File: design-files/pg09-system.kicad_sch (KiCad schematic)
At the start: 15 parts, among them U101 MC6809E, U102 GAL22V10, U103 74AHCT245, U104 74AHCT245, U105 74AHCT245, U106 GAL22V10

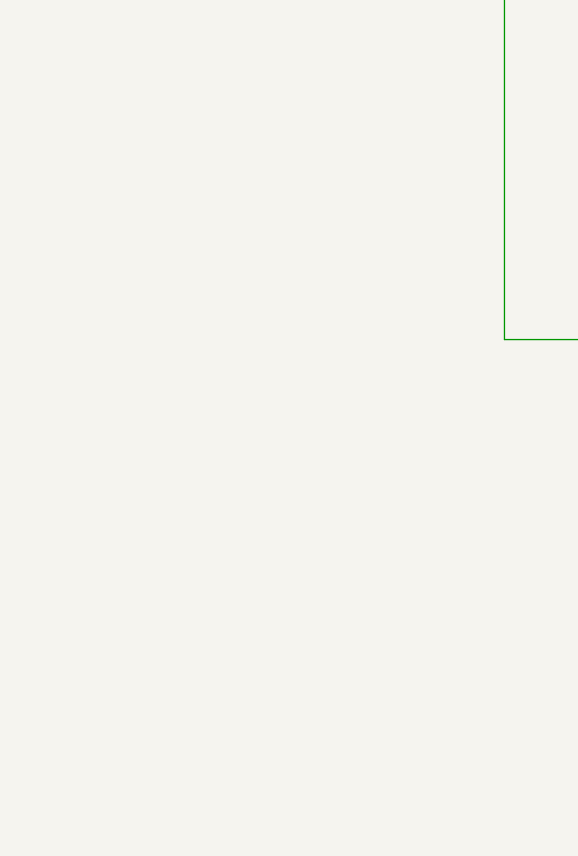
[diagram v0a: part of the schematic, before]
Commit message: Checkpoint WIP new PCB layout.
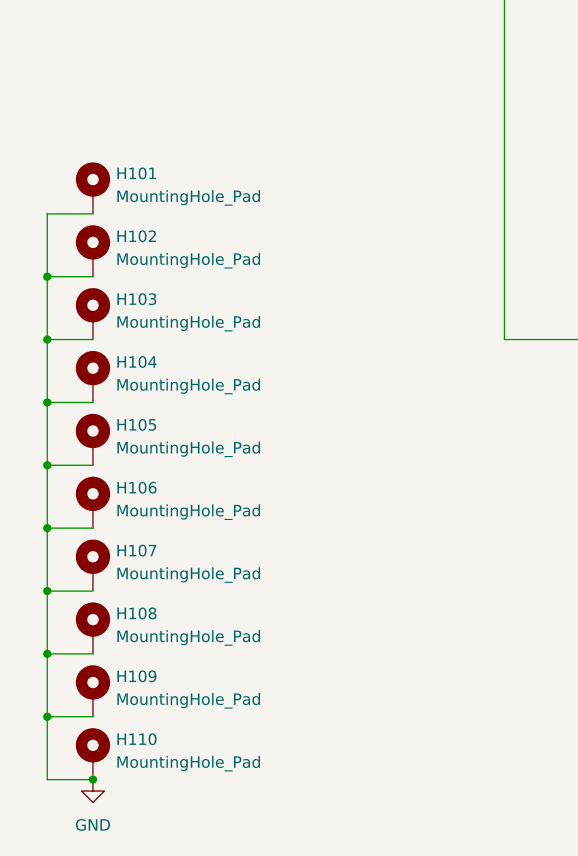
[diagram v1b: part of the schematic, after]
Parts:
- added H101, H102, H103, H104, H105, H106, H107, H108, H109, H110: MountingHole_Pad, MountingHole:MountingHole_4.3mm_M4_Pad_Via, symbol Mechanical:MountingHole_Pad
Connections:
- net GND: now also H101.1, H102.1, H103.1, H104.1, H105.1, H106.1, H107.1, H108.1, H109.1, H110.1
